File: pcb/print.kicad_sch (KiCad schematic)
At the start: 0 parts

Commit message: Initial commit
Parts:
- added C1, C10, C5, C6, C7, C8, C9: 100nF, Capacitor_SMD:C_0603_1608Metric, symbol Device:C_Small
- added C2, C3: 1uF, Capacitor_SMD:C_0603_1608Metric, symbol Device:C_Small
- added C4: 4,7uF1 16V, Capacitor_SMD:C_1206_3216Metric, symbol Device:C_Polarized_Small
- added D1, D2: 5V0, Diode_SMD:D_0603_1608Metric, symbol Device:D_TVS_Small
- added D3, D4, D5, D6: WS2812B, LED_SMD:LED_WS2812B_PLCC4_5.0x5.0mm_P3.2mm, symbol LED:WS2812B
- added F1: MFFSMF050, Fuse:Fuse_0603_1608Metric, symbol Device:Polyfuse_Small
- added J1: USB_leads, Connector_PinHeader_2.54mm:PinHeader_1x04_P2.54mm_Horizontal, symbol Connector:Conn_01x04_Socket
- added J2: TC2030-IDC-NL, Lib_TC2030-IDC-NL:TC2030-IDC-NL, symbol Lib_TC2030-IDC-NL:TC2030-IDC-NL
- added R1, R2, R3, R4: 1K0, Resistor_SMD:R_0603_1608Metric, symbol Device:R_Small
- added U1: FT232RL, Package_SO:SSOP-28_5.3x10.2mm_P0.65mm, symbol Interface_USB:FT232RL
- added U2: ATmega328-A, Package_QFP:TQFP-32_7x7mm_P0.8mm, symbol MCU_Microchip_ATmega:ATmega328-A
- added Y1: 16MHz, Crystal:Crystal_SMD_3225-4Pin_3.2x2.5mm, symbol Device:Crystal_GND24
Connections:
- new net: D3.2 (DOUT), D4.4 (DIN)
- new net: D3.4 (DIN), R4.2
- new net: D1.2 (A2), J1.2 (Pin_2), U1.16 (USBD-)
- new net: D2.2 (A2), J1.3 (Pin_3), U1.15 (USBD+)
- new net: C5.1, U1.2 (DTR)
- new net: D4.2 (DOUT), D5.4 (DIN)
- new net: D5.2 (DOUT), D6.4 (DIN)
- new net: R3.1, U2.32 (PD2)
- new net: C6.1, U2.20 (AREF)
- new net: R2.1, U2.31 (PD1)
- new net: U2.7 (XTAL1/PB6), Y1.3
- new net: U2.8 (XTAL2/PB7), Y1.1
- new net: F1.1, J1.1 (Pin_1)
- new net +5V: C1.2, C10.1, C2.1, C3.1, C4.1, C7.1, C8.1, C9.1, D3.1 (VDD), D4.1 (VDD), D5.1 (VDD), D6.1 (VDD), F1.2, J2.2 (VCC), R1.1, U1.20 (VCC), U1.4 (VCCIO), U2.18 (AVCC), U2.4 (VCC), U2.6 (VCC)
- new net DATA: R4.1, U2.10 (PD6)
- new net GND: C1.1, C10.2, C2.2, C3.2, C4.2, C6.2, C7.2, C8.2, C9.2, D1.1 (A1), D2.1 (A1), D3.3 (VSS), D4.3 (VSS), D5.3 (VSS), D6.3 (VSS), J1.4 (Pin_4), J2.6 (VDD), U1.18 (GND), U1.21 (GND), U1.25 (AGND), U1.26 (TEST), U1.7 (GND), U2.21 (GND), U2.3 (GND), U2.5 (GND), Y1.2, Y1.4
- new net MISO: J2.1 (MISO), U2.16 (PB4)
- new net MOSI: J2.4 (MOSI), U2.15 (PB3)
- new net RESET: C5.2, J2.5 (~{RESET}), R1.2, U2.29 (~{RESET}/PC6)
- new net RXD: R3.2, U1.1 (TXD)
- new net SCK: J2.3 (SCK), U2.17 (PB5)
- new net TXD: R2.2, U1.5 (RXD)
- no-connect marks 0 -> 31
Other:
- company: PouwerTronics -> (none)
- title: New Project -> DND Light

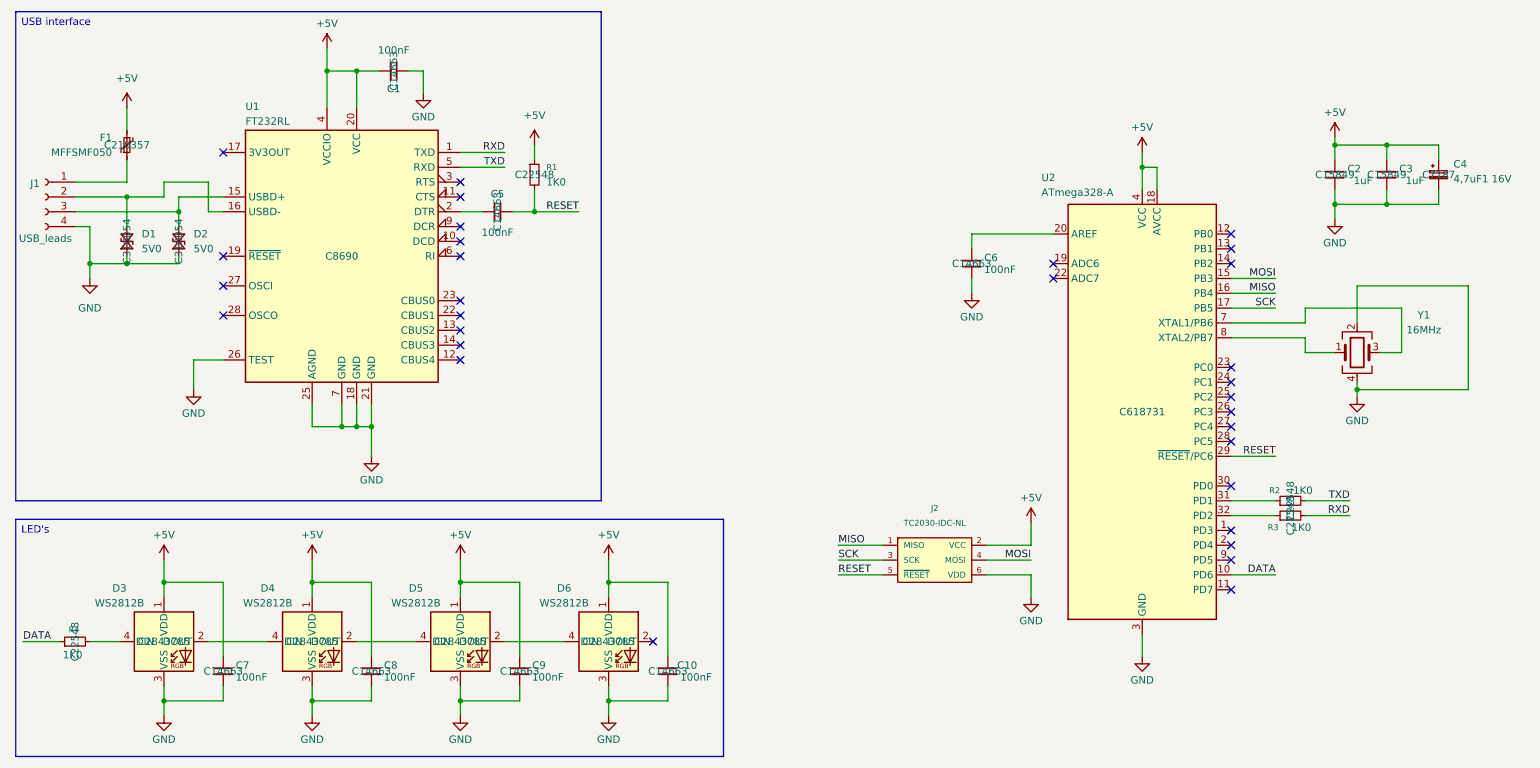
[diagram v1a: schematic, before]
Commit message: Add files via upload
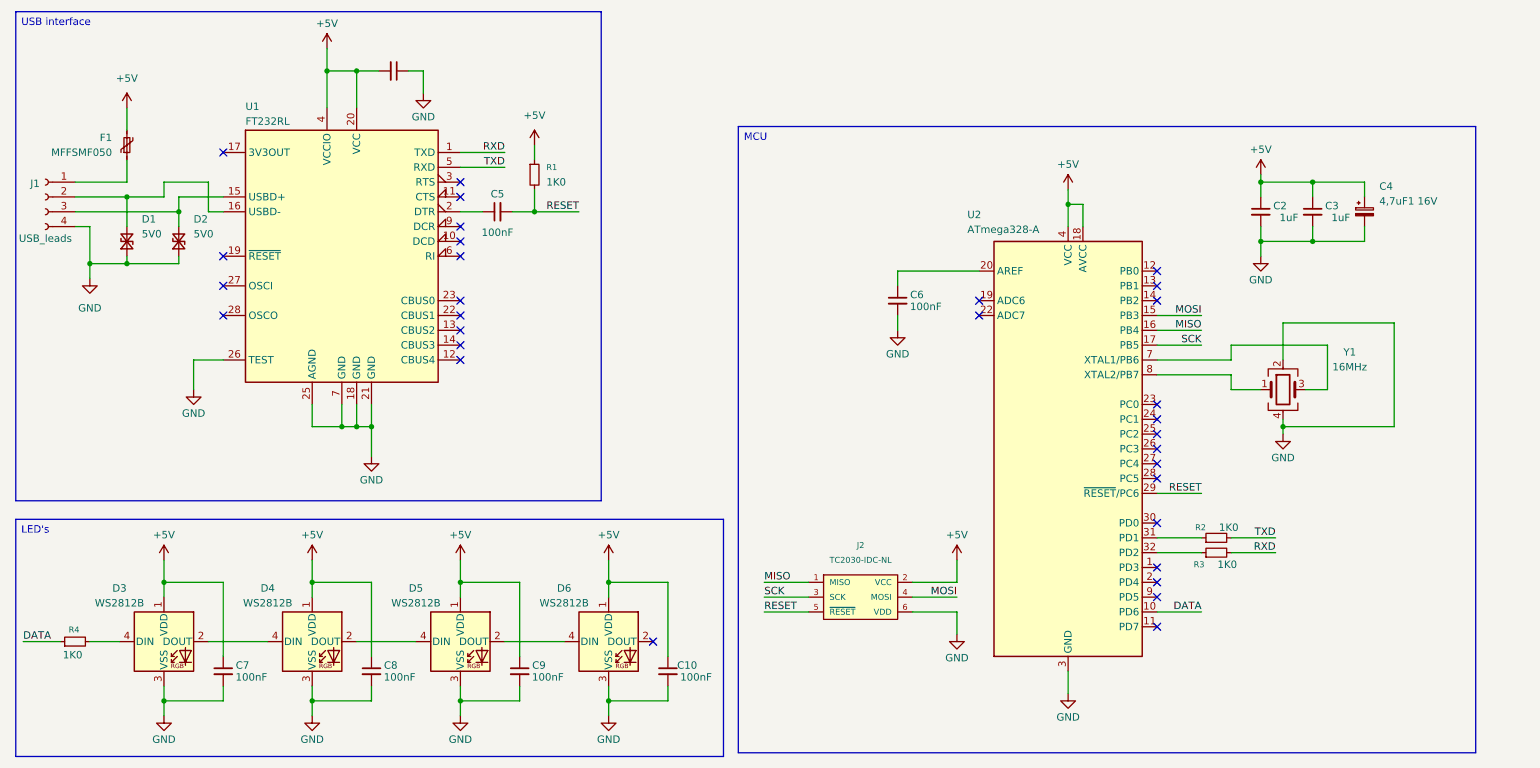
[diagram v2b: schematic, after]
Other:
- moved on the sheet: C2, C3, C4, C6, J2, R2, R3, U2, Y1

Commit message: Add files via upload
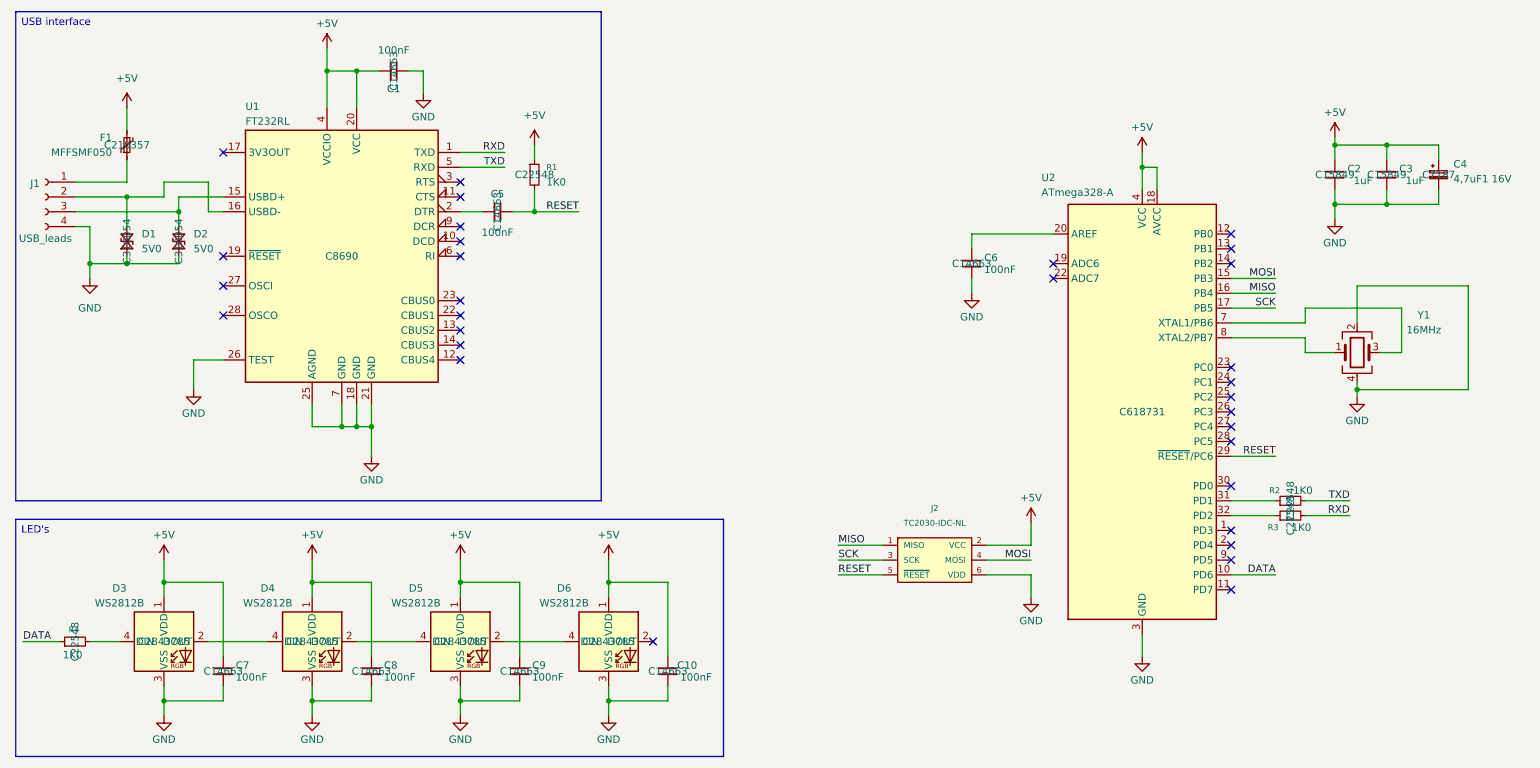
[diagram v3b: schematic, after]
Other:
- moved on the sheet: C2, C3, C4, C6, J2, R2, R3, U2, Y1
